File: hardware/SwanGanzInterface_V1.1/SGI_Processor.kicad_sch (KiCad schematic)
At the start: 31 parts, among them J2 Conn_01x08_Pin, SW2 MODE, SW3 ENTER, SW4 MODE, U4 XM0G3507QPTRQ1, U5 AdaFruit_1590, Y1 ABM8AIG-40.000MHZ-12-2Z-T3

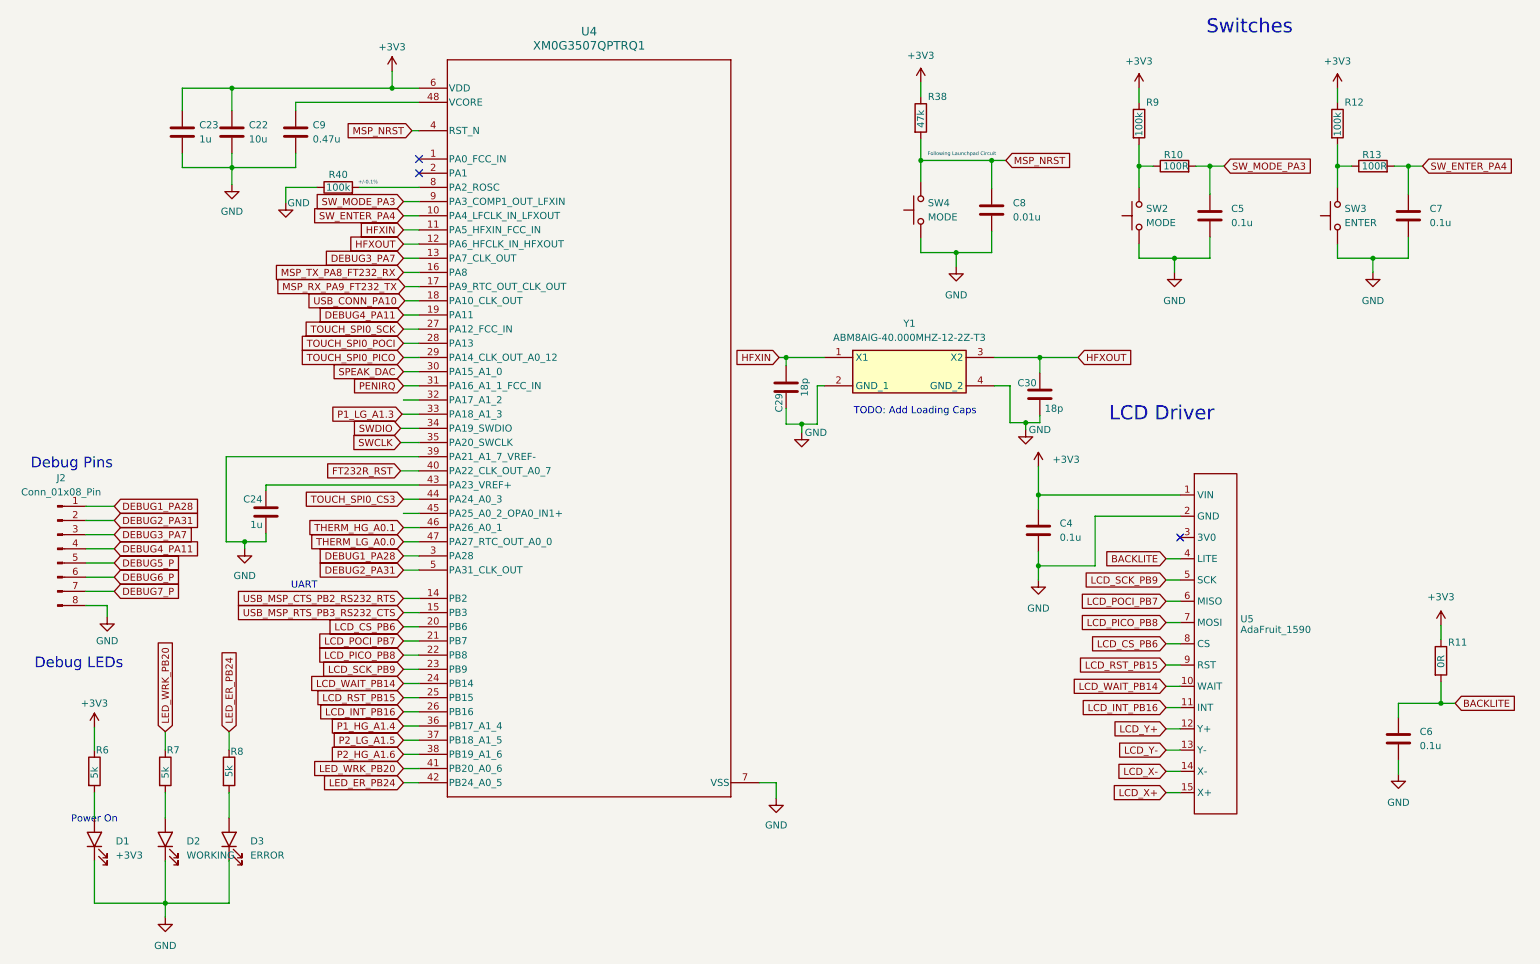
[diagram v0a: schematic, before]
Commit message: Added lots, moving to 64 pin micro
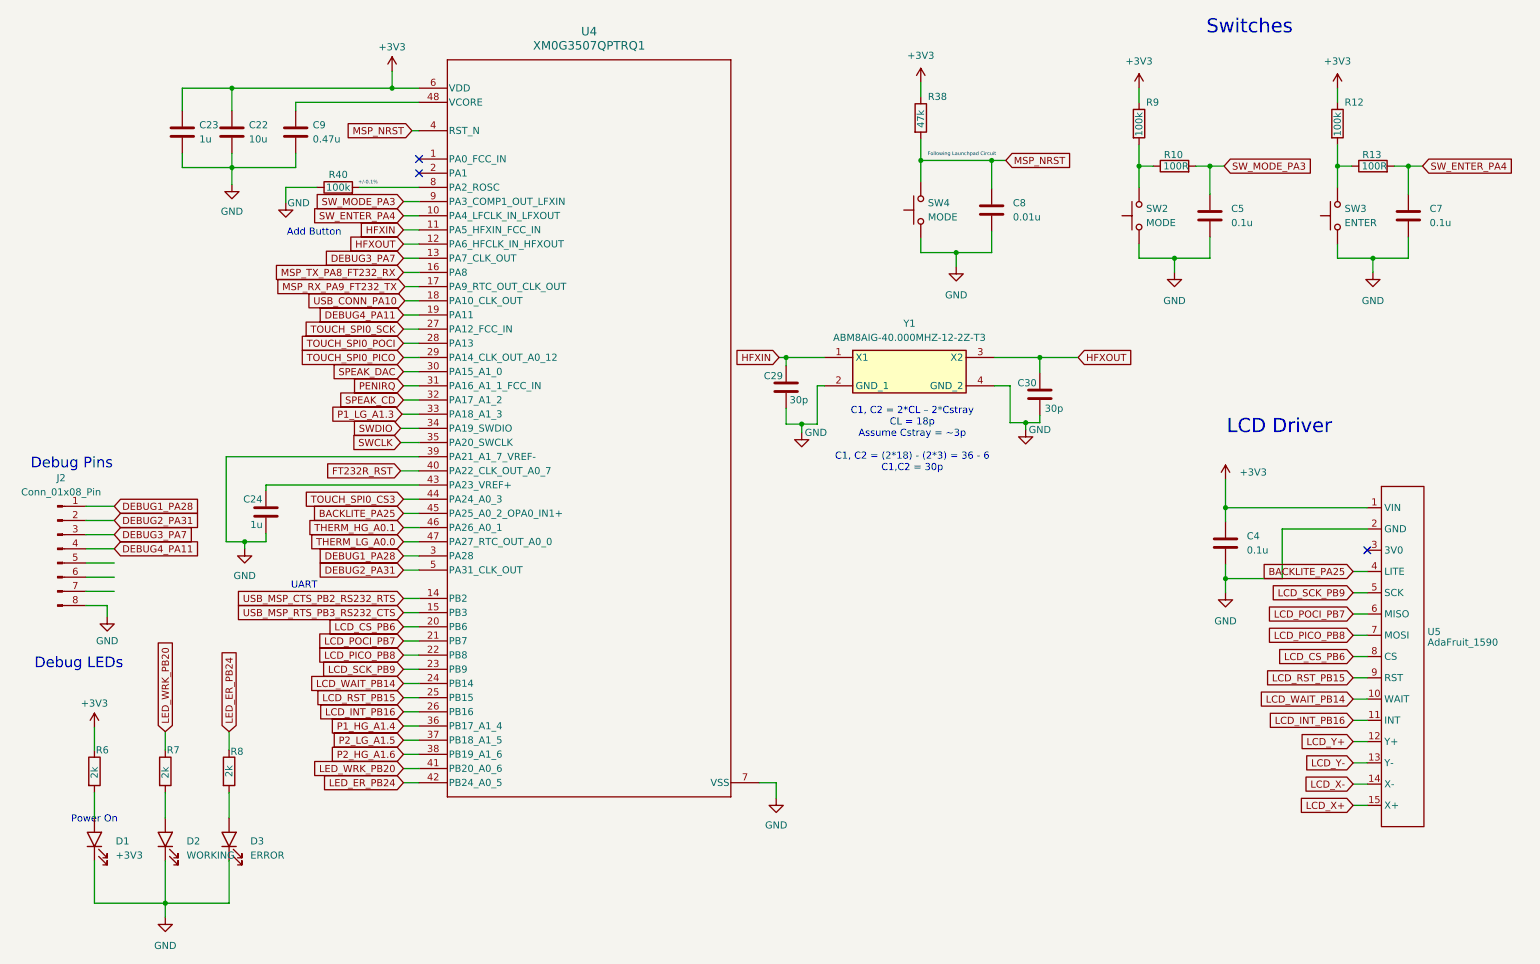
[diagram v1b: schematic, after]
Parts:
- removed C6: 0.1u, Capacitor_SMD:C_0603_1608Metric, symbol Device:C
- removed R11: 0R, Resistor_SMD:R_0603_1608Metric, symbol Device:R
- C29, C30: value 18p -> 30p
- R6, R7, R8: value 5k -> 2k
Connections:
- net BACKLITE is gone; now on net BACKLITE_PA25: U5.4 (LITE)
- net SPEAK_CD: now reaches U4.32 (PA17_A1_2)
- net BACKLITE_PA25: now reaches U4.45 (PA25_A0_2_OPA0_IN1+)
- net DEBUG5_P: no longer names the net of J2.5 (Pin_5)
- net DEBUG6_P: no longer names the net of J2.6 (Pin_6)
- net DEBUG7_P: no longer names the net of J2.7 (Pin_7)
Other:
- note added: "Add Button"
- note added: "C1, C2 = 2*CL – 2*Cstray CL = 18p Assume Cstray = ~3p C1, C2 = (2*18) - (2*3) = 36 - 6 C1,C2 = 30p"
- note removed: "TODO: Add Loading Caps"
- moved on the sheet: C4, U5
